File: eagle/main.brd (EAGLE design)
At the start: 49.2 x 49.5 mm, 43 parts, among them Q1 SQJ886EP, U1 LTC3789EGNPBF

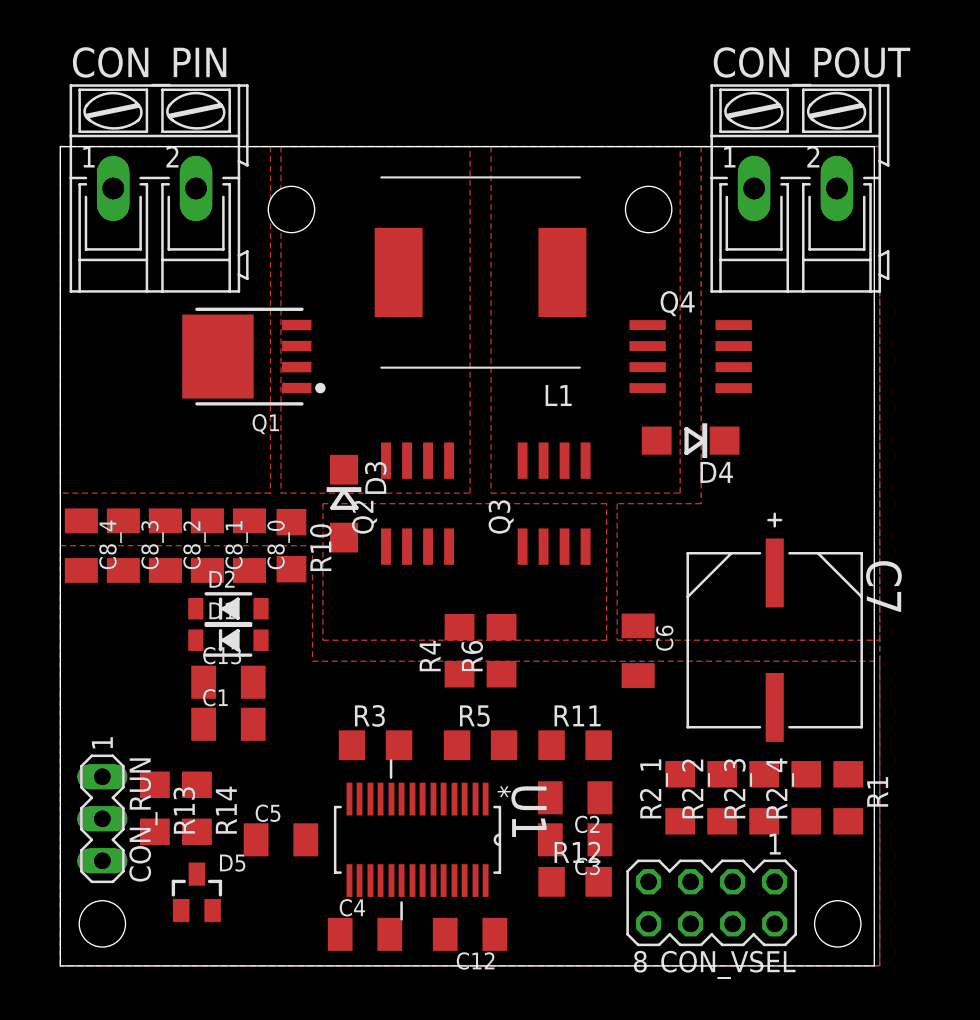
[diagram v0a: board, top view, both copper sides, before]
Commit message: [ update ] sch
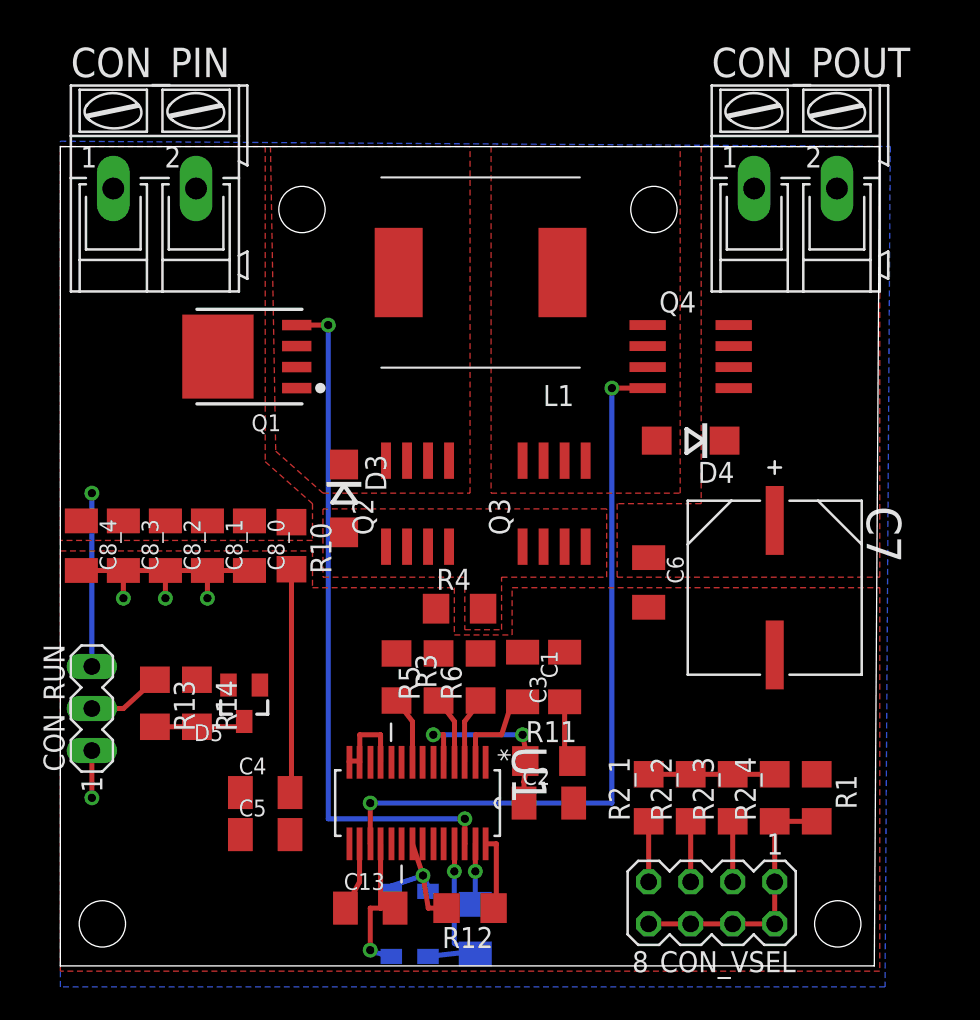
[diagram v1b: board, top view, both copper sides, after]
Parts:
- moved D2 21.4 mm to (20.0, 2.54), flipped to the bottom, turned to 90 degrees
- moved D1 21.0 mm to (22.2, 2.54), flipped to the bottom, turned to 90 degrees
- moved C1 18.0 mm to (27.9, 17.5), turned to 270 degrees
- moved C13 16.1 mm to (18.7, 3.49)
- moved D5 11.8 mm to (11.1, 15.9), turned to 180 degrees
- moved C4 10.5 mm to (12.4, 10.5)
- moved C3 9.86 mm to (30.5, 17.5), turned to 90 degrees
- moved CON_RUN 6.70 mm to (1.91, 15.6), turned to 90 degrees
- moved R12 6.55 mm to (24.8, 3.49), turned to 180 degrees
- moved R13 6.35 mm to (5.71, 15.9)
- moved R14 6.35 mm to (8.26, 15.9)
- moved R5 4.85 mm to (22.9, 17.5), turned to 90 degrees
- moved R3 4.32 mm to (20.3, 17.5), turned to 270 degrees
- moved C6 4.18 mm to (35.6, 23.2)
- moved C7 3.18 mm to (43.2, 22.9)
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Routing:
- net TG2: track 0.00 -> 44.3 mm, vias 0 -> 2
- net TG1: track 0.00 -> 41.5 mm, vias 0 -> 2
- net GND: track 0.00 -> 18.0 mm, vias 0 -> 4
- net VFB: track 0.00 -> 16.4 mm
- net N$2: track 0.00 -> 13.6 mm
- net N$4: track 0.00 -> 13.1 mm, vias 0 -> 2
- net VOUT: track 0.00 -> 13.0 mm
- net BOOST1: track 0.00 -> 10.5 mm, vias 0 -> 1
- net VIN: track 0.00 -> 10.5 mm, vias 0 -> 1
- net BOOST2: track 0.00 -> 9.30 mm, vias 0 -> 1
- net INTVCC: track 0.00 -> 8.48 mm, vias 0 -> 1
- net N$3: track 0.00 -> 5.96 mm
- net RUN: track 0.00 -> 5.72 mm
- net N$6: track 0.00 -> 4.70 mm
- net N$11: track 0.00 -> 4.48 mm
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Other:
- board size 49.2 x 49.5 mm -> 49.5 x 49.5 mm

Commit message: [ update ] sch
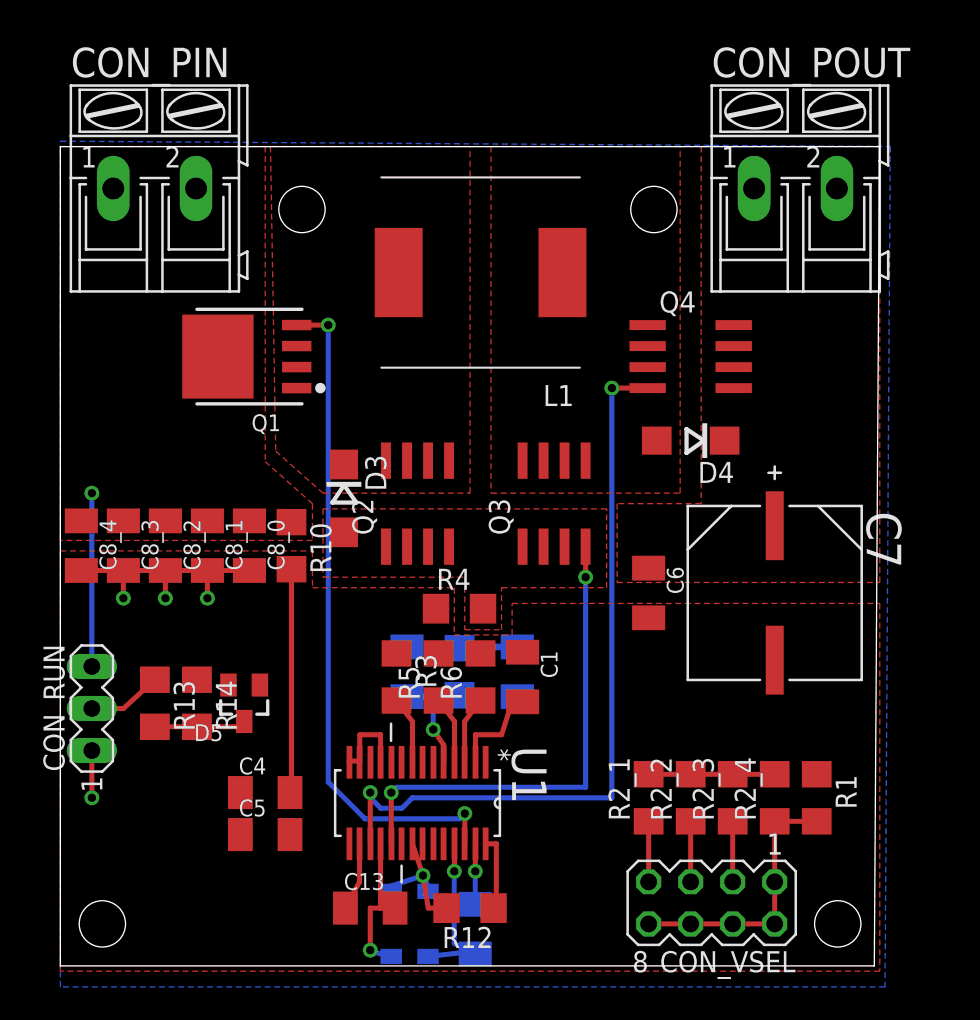
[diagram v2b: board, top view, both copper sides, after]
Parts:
- moved C2 11.7 mm to (21.0, 17.8), flipped to the bottom, turned to 90 degrees
- moved R11 7.63 mm to (24.1, 17.8), flipped to the bottom, turned to 90 degrees
- moved C3 2.88 mm to (27.6, 17.8), flipped to the bottom, turned to 270 degrees
- moved C6 0.63 mm to (35.6, 22.5)
- moved C7 0.32 mm to (43.2, 22.5)
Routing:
- net BG2: track 0.00 -> 29.5 mm, vias 0 -> 2
- net N$4: track 13.1 -> 7.43 mm, vias 2 -> 1
- net TG2: track 44.3 -> 45.5 mm
- net TG1: track 41.5 -> 40.7 mm
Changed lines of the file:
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@@
 <element name="R10" library="resistor" package="R1206" value="10" x="13.97" y="25.4" rot="R270"/>
 <element name="C1" library="rcl" package="C1206K" value="6.8n" x="27.94" y="17.4625" rot="R270"/>
-<element name="R11" library="resistor" package="R1206" value="68K" x="29.5275" y="12.3825"/>
-<element name="C2" library="rcl" package="C1206K" value="1n" x="29.5275" y="9.8425"/>
-<element name="C3" library="rcl" package="C1206K" value="3.3n" x="30.48" y="17.4625" rot="R90"/>
+<element name="R11" library="resistor" package="R1206" value="68K" x="24.13" y="17.78" rot="MR90"/>
+<element name="C2" library="rcl" package="C1206K" value="1n" x="20.955" y="17.78" rot="MR90"/>
+<element name="C3" library="rcl" package="C1206K" value="3.3n" x="27.6225" y="17.78" rot="MR270"/>
 <element name="C4" library="rcl" package="C1206K" value="1u" x="12.3825" y="10.4775"/>
 <element name="C5" library="rcl" package="C1206K" value="4.7u" x="12.3825" y="7.9375"/>
-<element name="C6" library="rcl" package="C1206K" value="2.2u" x="35.56" y="23.1775" rot="R270"/>
+<element name="C6" library="rcl" package="C1206K" value="2.2u" x="35.56" y="22.5425" rot="R270"/>
 <element name="C8_0" library="rcl" package="C1206K" value="10u" x="11.43" y="25.4" rot="R270"/>
 <element name="C12" library="rcl" package="C1206K" value="0.22u" x="25.0825" y="2.2225" rot="MR270"/>
@@
 <element name="Q4" library="transistor-power" package="SO-08" value="" x="38.1" y="36.83" rot="R270"/>
 <element name="Q1" library="transistor-fet" package="POWERPAK-SO-08" value="SQJ886EP" x="11.43" y="36.83" rot="R90"/>
-<element name="C7" library="Panasonic-EEEFT_EEEH" package="CAPAE1030X1050N" value="330UF" x="43.18" y="22.86" rot="R270">
-<attribute name="PACKAGE" value="CASE-G" x="43.18" y="22.86" size="1.778" layer="27" rot="R270" display="off"/>
-<attribute name="OC_NEWARK" value="31T8184" x="43.18" y="22.86" size="1.778" layer="27" rot="R270" display="off"/>
-<attribute name="TOLERANCE" value="±20 %" x="43.18" y="22.86" size="1.778" layer="27" rot="R270" display="off"/>
-<attribute name="MPN" value="EEE-FT1H331AP" x="43.18" y="22.86" size="1.778" layer="27" rot="R270" display="off"/>
-<attribute name="SUPPLIER" value="PANASONIC" x="43.18" y="22.86" size="1.778" layer="27" rot="R270" display="off"/>
-<attribute name="VOLTAGERATING" value="50V" x="43.18" y="22.86" size="1.778" layer="27" rot="R270" display="off"/>
-<attribute name="OC_FARNELL" value="1868428  " x="43.18" y="22.86" size="1.778" layer="27" rot="R270" display="off"/>
+<element name="C7" library="Panasonic-EEEFT_EEEH" package="CAPAE1030X1050N" value="330UF" x="43.18" y="22.5425" rot="R270">
+<attribute name="PACKAGE" value="CASE-G" x="43.18" y="22.5425" size="1.778" layer="27" rot="R270" display="off"/>
+<attribute name="OC_NEWARK" value="31T8184" x="43.18" y="22.5425" size="1.778" layer="27" rot="R270" display="off"/>
+<attribute name="TOLERANCE" value="±20 %" x="43.18" y="22.5425" size="1.778" layer="27" rot="R270" display="off"/>
+<attribute name="MPN" value="EEE-FT1H331AP" x="43.18" y="22.5425" size="1.778" layer="27" rot="R270" display="off"/>
+<attribute name="SUPPLIER" value="PANASONIC" x="43.18" y="22.5425" size="1.778" layer="27" rot="R270" display="off"/>
+<attribute name="VOLTAGERATING" value="50V" x="43.18" y="22.5425" size="1.778" layer="27" rot="R270" display="off"/>
+<attribute name="OC_FARNELL" value="1868428  " x="43.18" y="22.5425" size="1.778" layer="27" rot="R270" display="off"/>
 </element>
 <element name="C8_1" library="rcl" package="C1206K" value="10u" x="8.89" y="25.4" rot="R270"/>
@@
 <vertex x="23.8125" y="20.0025"/>
 <vertex x="27.305" y="20.0025"/>
-<vertex x="27.305" y="22.86"/>
-<vertex x="49.53" y="22.86"/>
+<vertex x="27.305" y="21.9075"/>
+<vertex x="49.53" y="21.9075"/>
 <vertex x="49.53" y="-0.3175"/>
 </polygon>
@@
 <vertex x="38.735" y="27.94"/>
 <vertex x="33.655" y="27.94"/>
-<vertex x="33.655" y="23.495"/>
-<vertex x="49.53" y="23.495"/>
+<vertex x="33.655" y="23.1775"/>
+<vertex x="49.53" y="23.1775"/>
 <vertex x="49.53" y="49.53"/>
 </polygon>
@@
 <wire x1="18.0975" y1="13.97" x2="19.3548" y2="13.97" width="0.3048" layer="1"/>
 <wire x1="19.3548" y1="13.97" x2="19.3548" y2="12.3063" width="0.3048" layer="1"/>
-<wire x1="35.56" y1="24.6775" x2="35.56" y2="11.582" width="0" layer="19" extent="1-1"/>
+<wire x1="35.56" y1="24.0425" x2="35.56" y2="11.582" width="0" layer="19" extent="1-1"/>
 <wire x1="20.6248" y1="7.3787" x2="35.56" y2="11.582" width="0" layer="19" extent="1-1"/>
 <wire x1="19.3548" y1="12.3063" x2="20.6248" y2="7.3787" width="0" layer="19" extent="1-1"/>
@@
 <contactref element="R11" pad="1"/>
 <contactref element="C2" pad="1"/>
-<wire x1="28.0275" y1="9.8425" x2="28.0275" y2="11.1125" width="0.3048" layer="1"/>
-<wire x1="28.0275" y1="11.1125" x2="28.2575" y2="12.3825" width="0.3048" layer="1"/>
-<wire x1="28.2575" y1="12.3825" x2="27.94" y2="13.97" width="0.3048" layer="1"/>
-<via x="27.94" y="13.97" extent="1-16" drill="0.5"/>
-<wire x1="27.94" y1="13.97" x2="22.5425" y2="13.97" width="0.3048" layer="16"/>
-<via x="22.5425" y="13.97" extent="1-16" drill="0.5"/>
-<wire x1="22.5425" y1="13.97" x2="23.1648" y2="13.97" width="0.3048" layer="1"/>
-<wire x1="23.1648" y1="13.97" x2="23.1648" y2="12.3063" width="0.3048" layer="1"/>
-<wire x1="28.0275" y1="11.1125" x2="28.1055" y2="12.3825" width="0.3048" layer="1"/>
+<wire x1="20.955" y1="16.28" x2="22.5425" y2="16.28" width="0.4064" layer="16"/>
+<wire x1="22.5425" y1="16.28" x2="24.13" y2="16.28" width="0.4064" layer="16"/>
+<wire x1="24.13" y1="16.28" x2="24.13" y2="16.358" width="0.4064" layer="16"/>
+<wire x1="23.1648" y1="12.3063" x2="23.1775" y2="12.3063" width="0.3048" layer="1"/>
+<wire x1="23.1775" y1="12.3063" x2="23.1775" y2="13.335" width="0.3048" layer="1"/>
+<wire x1="23.1775" y1="13.335" x2="22.5425" y2="14.2875" width="0.3048" layer="1"/>
+<via x="22.5425" y="14.2875" extent="1-16" drill="0.5"/>
+<wire x1="22.5425" y1="14.2875" x2="22.5425" y2="16.28" width="0.3048" layer="16"/>
 </signal>
 <signal name="N$5">
 <contactref element="R11" pad="2"/>
 <contactref element="C3" pad="1"/>
-<wire x1="30.48" y1="15.9625" x2="30.48" y2="12.3825" width="0.3048" layer="1"/>
-<wire x1="30.48" y1="12.3825" x2="30.9495" y2="12.3825" width="0.3048" layer="1"/>
+<wire x1="27.6225" y1="19.28" x2="24.13" y2="19.28" width="0.4064" layer="16"/>
+<wire x1="24.13" y1="19.28" x2="24.13" y2="19.202" width="0.4064" layer="16"/>
 </signal>
 <signal name="BOOST1">
@@
 <wire x1="35.5" y1="34.925" x2="33.3375" y2="34.925" width="0.3048" layer="1"/>
 <via x="33.3375" y="34.925" extent="1-16" drill="0.5"/>
-<wire x1="33.3375" y1="34.925" x2="33.3375" y2="9.8425" width="0.3048" layer="16"/>
-<wire x1="33.3375" y1="9.8425" x2="18.7325" y2="9.8425" width="0.3048" layer="16"/>
-<via x="18.7325" y="9.8425" extent="1-16" drill="0.5"/>
-<wire x1="18.7325" y1="9.8425" x2="18.7325" y2="7.3787" width="0.3048" layer="1"/>
+<wire x1="33.3375" y1="34.925" x2="33.3375" y2="10.16" width="0.3048" layer="16"/>
+<wire x1="33.3375" y1="10.16" x2="21.2725" y2="10.16" width="0.3048" layer="16"/>
+<wire x1="21.2725" y1="10.16" x2="20.6375" y2="9.525" width="0.3048" layer="16"/>
+<wire x1="20.6375" y1="9.525" x2="19.3675" y2="9.525" width="0.3048" layer="16"/>
+<wire x1="19.3675" y1="9.525" x2="18.7325" y2="10.16" width="0.3048" layer="16"/>
+<wire x1="18.7325" y1="10.16" x2="18.7325" y2="10.4775" width="0.3048" layer="16"/>
+<via x="18.7325" y="10.4775" extent="1-16" drill="0.5"/>
+<wire x1="18.7325" y1="10.4775" x2="18.7325" y2="7.3787" width="0.3048" layer="1"/>
 <wire x1="18.7325" y1="7.3787" x2="18.7452" y2="7.3787" width="0.3048" layer="1"/>
 </signal>
@@
 <wire x1="14.2875" y1="38.735" x2="16.1925" y2="38.735" width="0.3048" layer="1"/>
 <via x="16.1925" y="38.735" extent="1-16" drill="0.5"/>
-<wire x1="16.1925" y1="38.735" x2="16.1925" y2="8.89" width="0.3048" layer="16"/>
-<wire x1="16.1925" y1="8.89" x2="24.4475" y2="8.89" width="0.3048" layer="16"/>
-<via x="24.4475" y="8.89" extent="1-16" drill="0.5"/>
-<wire x1="24.4475" y1="8.89" x2="24.4475" y2="7.3787" width="0.3048" layer="1"/>
+<wire x1="16.1925" y1="38.735" x2="16.1925" y2="11.1125" width="0.3048" layer="16"/>
+<wire x1="16.1925" y1="11.1125" x2="18.415" y2="8.89" width="0.3048" layer="16"/>
+<wire x1="18.415" y1="8.89" x2="24.13" y2="8.89" width="0.3048" layer="16"/>
+<wire x1="24.13" y1="8.89" x2="24.4475" y2="9.2075" width="0.3048" layer="16"/>
+<via x="24.4475" y="9.2075" extent="1-16" drill="0.5"/>
+<wire x1="24.4475" y1="9.2075" x2="24.4475" y2="7.3787" width="0.3048" layer="1"/>
 <wire x1="24.4475" y1="7.3787" x2="24.4348" y2="7.3787" width="0.3048" layer="1"/>
 </signal>
@@
 <contactref element="U1" pad="19"/>
 <contactref element="Q3" pad="4"/>
-<wire x1="20.0152" y1="7.3787" x2="31.75" y2="25.34" width="0" layer="19" extent="1-1"/>
+<wire x1="20.0152" y1="7.3787" x2="20.0025" y2="7.3787" width="0.3048" layer="1"/>
+<wire x1="20.0025" y1="7.3787" x2="20.0025" y2="10.4775" width="0.3048" layer="1"/>
+<via x="20.0025" y="10.4775" extent="1-16" drill="0.5"/>
+<wire x1="20.0025" y1="10.4775" x2="20.32" y2="10.795" width="0.3048" layer="16"/>
+<wire x1="20.32" y1="10.795" x2="31.75" y2="10.795" width="0.3048" layer="16"/>
+<wire x1="31.75" y1="10.795" x2="31.75" y2="23.495" width="0.3048" layer="16"/>
+<via x="31.75" y="23.495" extent="1-16" drill="0.5"/>
+<wire x1="31.75" y1="23.495" x2="31.75" y2="25.34" width="0.3048" layer="1"/>
 </signal>
 <signal name="BG1">
@@
 <vertex x="24.4475" y="20.32"/>
 <vertex x="26.67" y="20.32"/>
-<vertex x="26.67" y="23.495"/>
-<vertex x="33.02" y="23.495"/>
+<vertex x="26.67" y="22.86"/>
+<vertex x="33.02" y="22.86"/>
 <vertex x="33.02" y="27.6225"/>
 <vertex x="15.875" y="27.6225"/>

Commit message: [ update ] sch
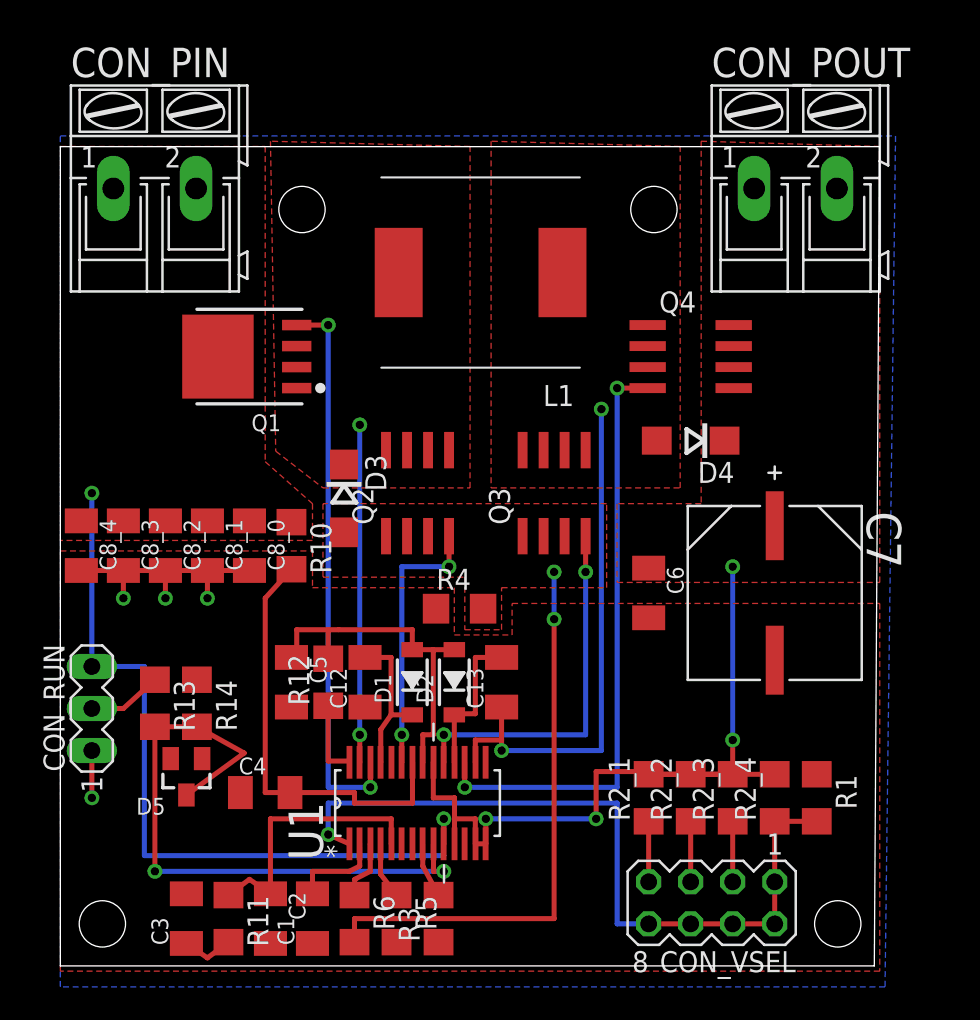
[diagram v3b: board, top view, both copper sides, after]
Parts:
- moved C3 25.0 mm to (7.62, 2.86), flipped to the top, turned to 90 degrees
- moved R11 20.4 mm to (10.2, 2.86), flipped to the top, turned to 270 degrees
- moved C1 19.4 mm to (15.2, 2.86), turned to 90 degrees
- moved C2 17.1 mm to (12.7, 2.86), flipped to the top, turned to 270 degrees
- moved R6 16.5 mm to (17.8, 2.86), turned to 270 degrees
- moved C12 16.3 mm to (18.4, 17.1), flipped to the top, turned to 90 degrees
- moved R12 16.1 mm to (16.2, 17.1), turned to 90 degrees
- moved C13 15.8 mm to (26.7, 17.1), turned to 90 degrees
- moved D2 15.1 mm to (23.8, 17.1), flipped to the top
- moved R3 14.8 mm to (22.9, 2.86), turned to 90 degrees
- moved R5 14.8 mm to (20.3, 2.86), turned to 270 degrees
- moved D1 14.6 mm to (21.3, 17.1), flipped to the top
- moved C5 9.34 mm to (14.0, 17.1), turned to 270 degrees
- moved D5 5.65 mm to (7.62, 11.4)
- moved Q2 0.63 mm to (21.6, 28.6)
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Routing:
- net VIN: track 10.5 -> 46.9 mm, vias 1 -> 2
- net VOUT: track 13.0 -> 49.3 mm, vias 0 -> 4
- net N$9: track 0.00 -> 34.4 mm, vias 0 -> 2
- net RUN: track 5.72 -> 38.6 mm, vias 0 -> 2
- net VFB: track 16.4 -> 46.3 mm, vias 0 -> 1
- net SW2: track 4.10 -> 32.2 mm, vias 0 -> 2
- net SW1: track 3.67 -> 20.4 mm, vias 1 -> 2
- net BG1: track 0.00 -> 16.5 mm, vias 0 -> 2
- net INTVCC: track 8.48 -> 21.9 mm, vias 1 -> 0
- net N$2: track 13.6 -> 26.1 mm
- net N$4: track 7.43 -> 16.5 mm, vias 1 -> 0
- net TG2: track 45.5 -> 36.7 mm
- net BG2: track 29.5 -> 22.3 mm
- net TG1: track 40.7 -> 33.9 mm
- net BOOST1: track 10.5 -> 9.41 mm, vias 1 -> 0
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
